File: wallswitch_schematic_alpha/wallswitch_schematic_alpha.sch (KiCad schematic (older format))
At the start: 60 parts, among them IC1 HLW8012, J1 Conn_01x06, J2 Screw_Terminal_01x02, J3 Screw_Terminal_01x03, K1 SANYOU_SRD_Form_C, Q1 BC817DPN, Q2 2N7002, Q3 2N7002, SW1 SW_BOOT, SW2 SW_RESET, U1 AMS1117-3.3, U2 ESP32-WROOM-32D

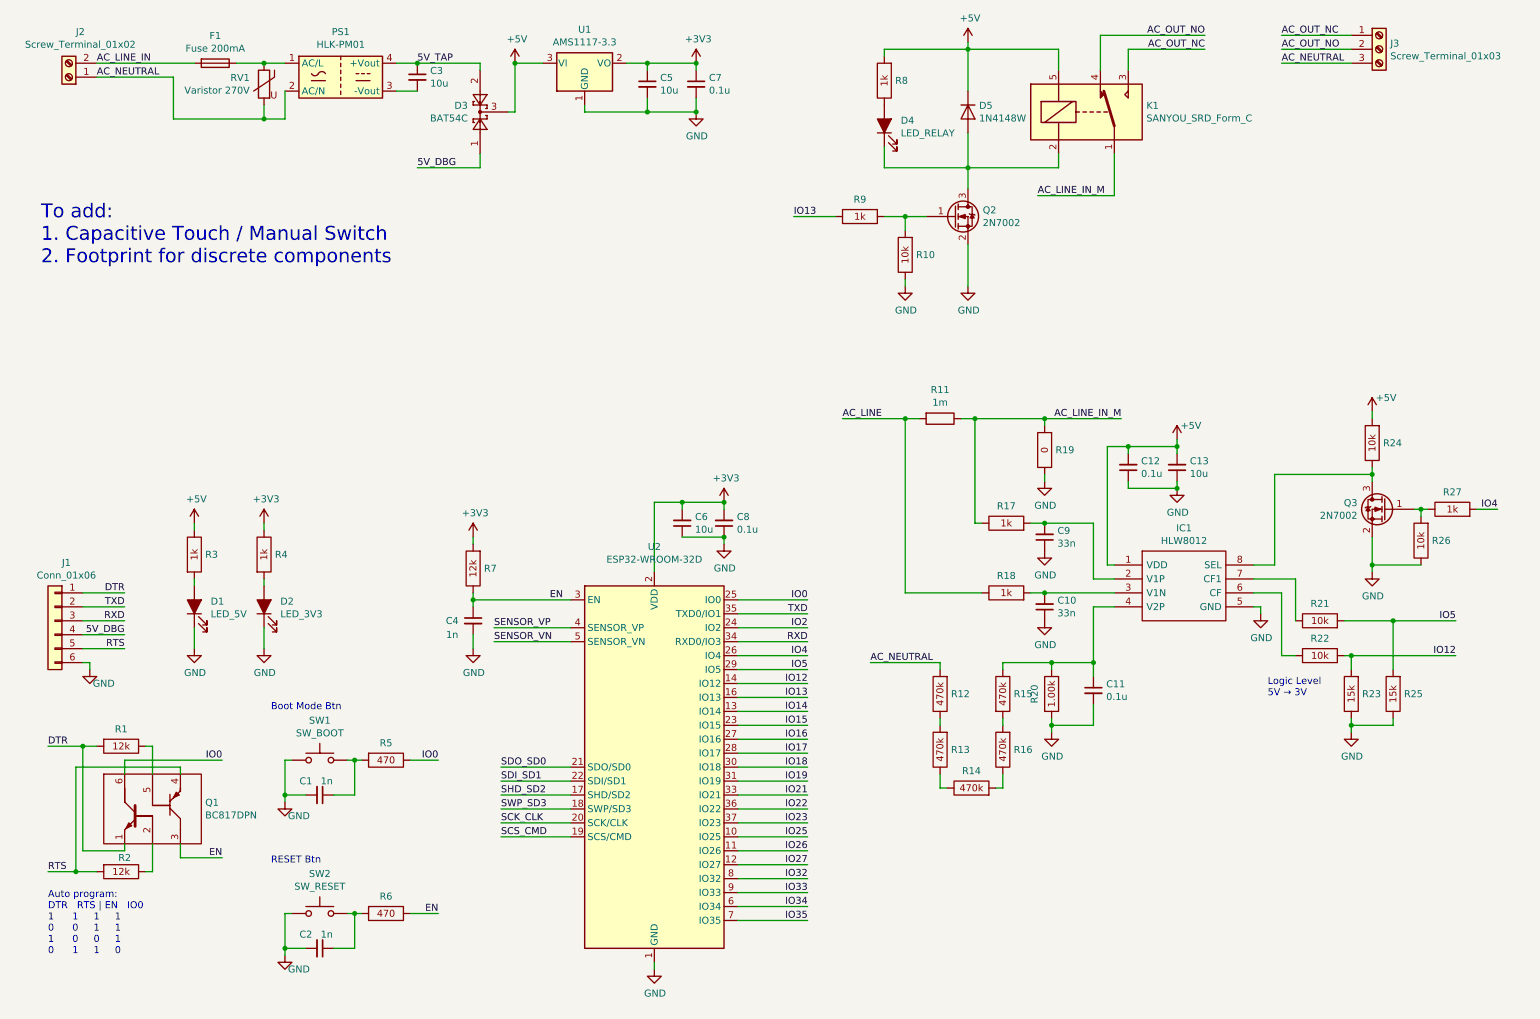
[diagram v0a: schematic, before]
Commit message: progress for layout
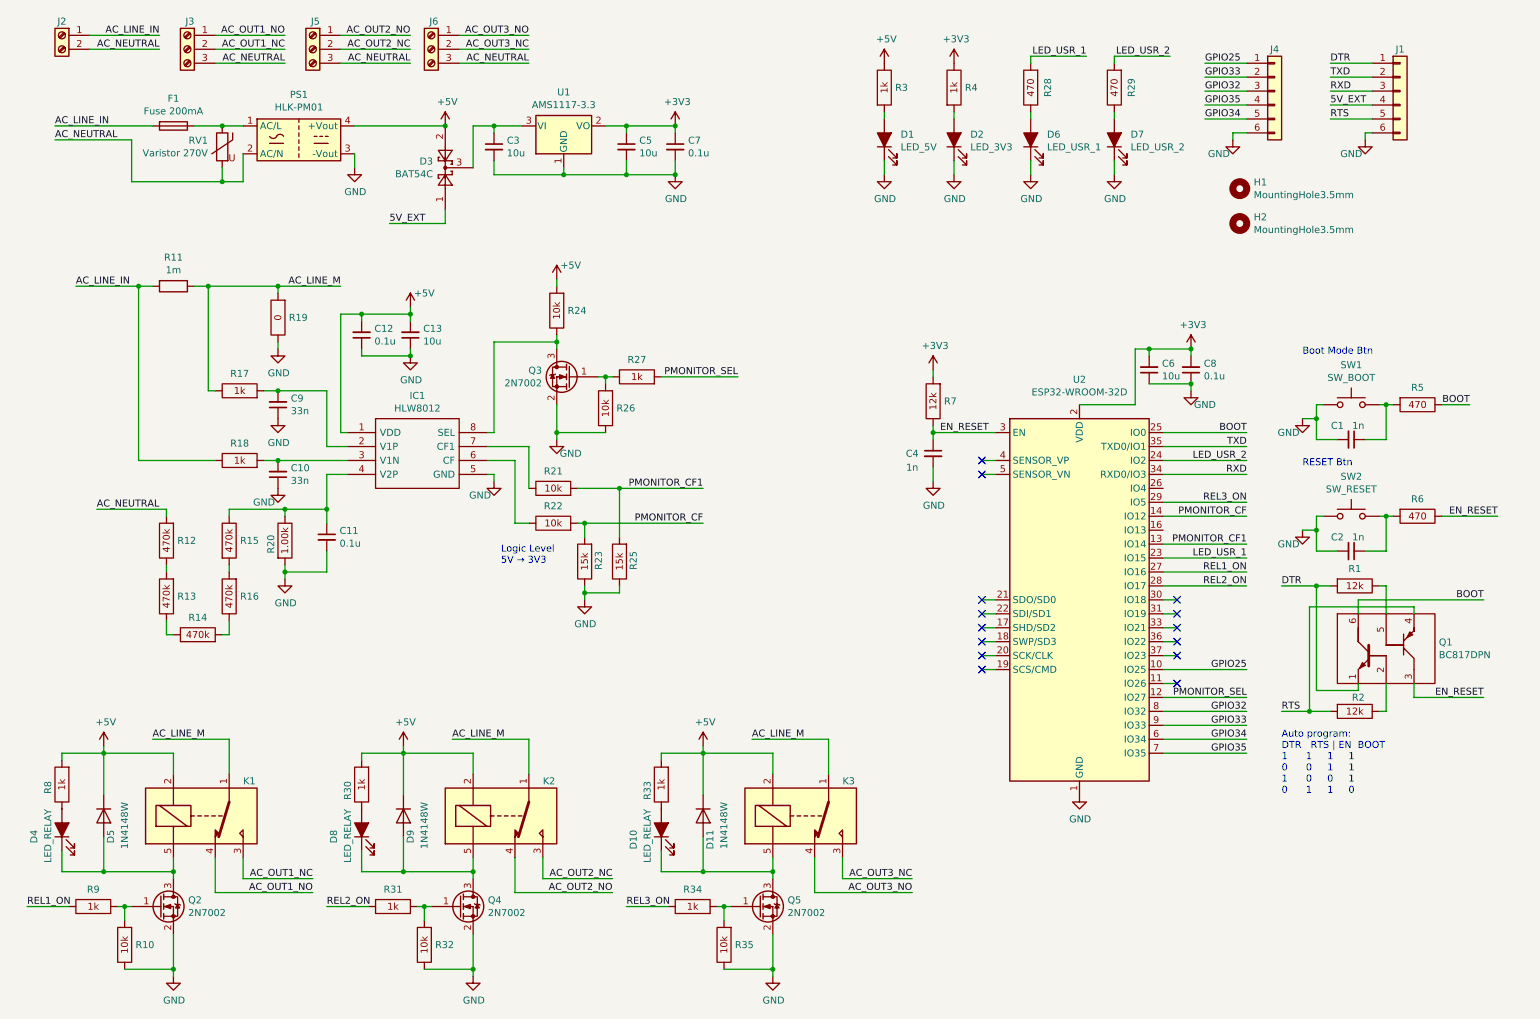
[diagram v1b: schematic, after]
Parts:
- added D10, D8: LED_RELAY, LED_SMD:LED_0603_1608Metric, symbol Device:LED_ALT
- added D11, D9: 1N4148W, Diode_SMD:D_SOD-123, symbol Diode:1N4148W
- added D6: LED_USR_1, LED_SMD:LED_0603_1608Metric, symbol Device:LED_ALT
- added D7: LED_USR_2, LED_SMD:LED_0603_1608Metric, symbol Device:LED_ALT
- added H1, H2: MountingHole3.5mm, MountingHole:MountingHole_3.5mm, symbol Mechanical:MountingHole
- added J4: Conn_01x06, Connector_PinHeader_2.54mm:PinHeader_1x06_P2.54mm_Vertical, symbol Connector_Generic:Conn_01x06
- added J5, J6: Screw_Terminal_01x03, TerminalBlock:TerminalBlock_bornier-3_P5.08mm, symbol Connector:Screw_Terminal_01x03
- added K2, K3: SANYOU_SRD_Form_C, XLAB_Block:Relay_SPDT_SANYOU_SRD_Series_Form_C, symbol XLAB_Block:SANYOU_SRD_Form_C
- added Q4, Q5: 2N7002, Package_TO_SOT_SMD:SOT-23, symbol Transistor_FET:2N7002
- added R28, R29: R_470_±5%_1608m, R_0603_1608Metric, symbol XLAB_Resistor:R_470_±5%_1608m
- added R30, R31, R33, R34: R_1k_±5%_1608m, R_0603_1608Metric, symbol XLAB_Resistor:R_1k_±5%_1608m
- added R32, R35: R_10k_±5%_1608m, R_0603_1608Metric, symbol XLAB_Resistor:R_10k_±5%_1608m
- C1, C10, C11, C12, C13, C2, C3, C4, C5, C6, C7, C8, C9: footprint (none) -> Capacitor_SMD:C_0603_1608Metric
- F1: footprint (none) -> Fuse:Fuse_Blade_Mini_directSolder
- R11: footprint (none) -> Resistor_SMD:R_2512_6332Metric_Pad1.52x3.35mm_HandSolder
- RV1: footprint (none) -> Varistor:RV_Disc_D12mm_W3.9mm_P7.5mm
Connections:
- net AC_LINE is gone; now on net AC_LINE_IN: R11.2, R18.2
- net +5V: now also D3.2, K1.2, PS1.4 (+Vout), D11.1 (K), D9.1 (K), K2.2, K3.2, R30.1, R33.1; no longer D3.3, K1.5, U1.3 (VI)
- net AC_LINE_IN: now also J2.1 (Pin_1); no longer J2.2 (Pin_2)
- net AC_NEUTRAL: now also J2.2 (Pin_2), J5.3 (Pin_3), J6.3 (Pin_3); no longer J2.1 (Pin_1)
- net GND: now also C3.2, PS1.3 (-Vout), D6.1 (K), D7.1 (K), J4.6 (Pin_6), Q4.2 (S), Q5.2 (S), R32.2, R35.2
- net at D4.1 (K), D5.2 (A), Q2.3 (D): now also K1.5; no longer K1.2
- net 5V_DBG renamed 5V_EXT
- removed net 5V_TAP: C3.1, D3.2, PS1.4 (+Vout)
- net AC_LINE_IN_M renamed AC_LINE_M
- net AC_LINE_M: now also K2.1, K3.1
- net AC_OUT_NC renamed AC_OUT1_NC
- net AC_OUT1_NC: now also J3.2 (Pin_2); no longer J3.1 (Pin_1)
- net AC_OUT_NO renamed AC_OUT1_NO
- net AC_OUT1_NO: now also J3.1 (Pin_1); no longer J3.2 (Pin_2)
- net EN renamed EN_RESET
- net IO0 renamed BOOT
- net IO12 renamed PMONITOR_CF
- net IO13: no longer names the net of U2.16 (IO13)
- net IO13: no longer R9.2
- net IO14 renamed PMONITOR_CF1
- net PMONITOR_CF1: now also R21.1, R25.1
- net IO15 renamed LED_USR_1
- net LED_USR_1: now also R28.1
- net IO16 renamed REL1_ON
- net REL1_ON: now also R9.2
- net IO17 renamed REL2_ON
- net REL2_ON: now also R31.2
- net IO18: no longer names the net of U2.30 (IO18)
- net IO19: no longer names the net of U2.31 (IO19)
- net IO2 renamed LED_USR_2
- net LED_USR_2: now also R29.1
- net IO21: no longer names the net of U2.33 (IO21)
- net IO22: no longer names the net of U2.36 (IO22)
- net IO23: no longer names the net of U2.37 (IO23)
- net IO25 renamed GPIO25
- net GPIO25: now also J4.1 (Pin_1)
- net IO26: no longer names the net of U2.11 (IO26)
- net IO27 renamed PMONITOR_SEL
- net PMONITOR_SEL: now also R27.1
- net IO32 renamed GPIO32
- net GPIO32: now also J4.3 (Pin_3)
- net IO33 renamed GPIO33
- net GPIO33: now also J4.2 (Pin_2)
- net IO34 renamed GPIO34
- net GPIO34: now also J4.5 (Pin_5)
- net IO35 renamed GPIO35
- net GPIO35: now also J4.4 (Pin_4)
- net IO4: no longer names the net of U2.26 (IO4)
- net IO4: no longer R27.1
- removed net IO5: R21.1, R25.1, U2.29 (IO5)
- net SCK_CLK: no longer names the net of U2.20 (SCK/CLK)
- net SCS_CMD: no longer names the net of U2.19 (SCS/CMD)
- net SDI_SD1: no longer names the net of U2.22 (SDI/SD1)
- net SDO_SD0: no longer names the net of U2.21 (SDO/SD0)
- net SENSOR_VN: no longer names the net of U2.5 (SENSOR_VN)
- net SENSOR_VP: no longer names the net of U2.4 (SENSOR_VP)
- net SHD_SD2: no longer names the net of U2.17 (SHD/SD2)
- net SWP_SD3: no longer names the net of U2.18 (SWP/SD3)
- new net: C3.1, D3.3, U1.3 (VI)
- new net: D6.2 (A), R28.2
- new net: D7.2 (A), R29.2
- new net: D8.1 (K), D9.2 (A), K2.5, Q4.3 (D)
- new net: D8.2 (A), R30.2
- new net: Q4.1 (G), R31.1, R32.1
- new net: D10.1 (K), D11.2 (A), K3.5, Q5.3 (D)
- new net: D10.2 (A), R33.2
- new net: Q5.1 (G), R34.1, R35.1
- new net AC_OUT2_NC: J5.2 (Pin_2), K2.3
- new net AC_OUT2_NO: J5.1 (Pin_1), K2.4
- new net AC_OUT3_NC: J6.2 (Pin_2), K3.3
- new net AC_OUT3_NO: J6.1 (Pin_1), K3.4
- new net REL3_ON: R34.2, U2.29 (IO5)
- no-connect marks 0 -> 14
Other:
- note added: "Auto program:\nDTR RTS | EN BOOT\n1 1 1 1\n0 0 1 1\n1 0 0 1\n0 1 1 0"
- note added: "Logic Level\n5V → 3V3"
- note removed: "Auto program:\nDTR RTS | EN IO0\n1 1 1 1\n0 0 1 1\n1 0 0 1\n0 1 1 0"
- note removed: "Logic Level\n5V → 3V"
- note removed: "To add:\n1. Capacitive Touch / Manual Switch\n2. Footprint for discrete components"
- moved on the sheet: C1, C10, C11, C12, C13, C2, C3, C4, C5, C6, C7, C8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
